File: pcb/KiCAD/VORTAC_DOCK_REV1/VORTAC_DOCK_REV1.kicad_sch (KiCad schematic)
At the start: 31 parts, among them J1 Conn_01x05, J10 Conn_01x03, J2 Conn_01x03, J3 PowerSolderPoint, J4 Conn_01x03, J5 Conn_01x04, J6 Conn_01x04, J7 Conn_01x01, J8 Conn_01x01, J9 Conn_01x03, U1 WS2811, U2 TPS26630RGE, U6 AP63205WU

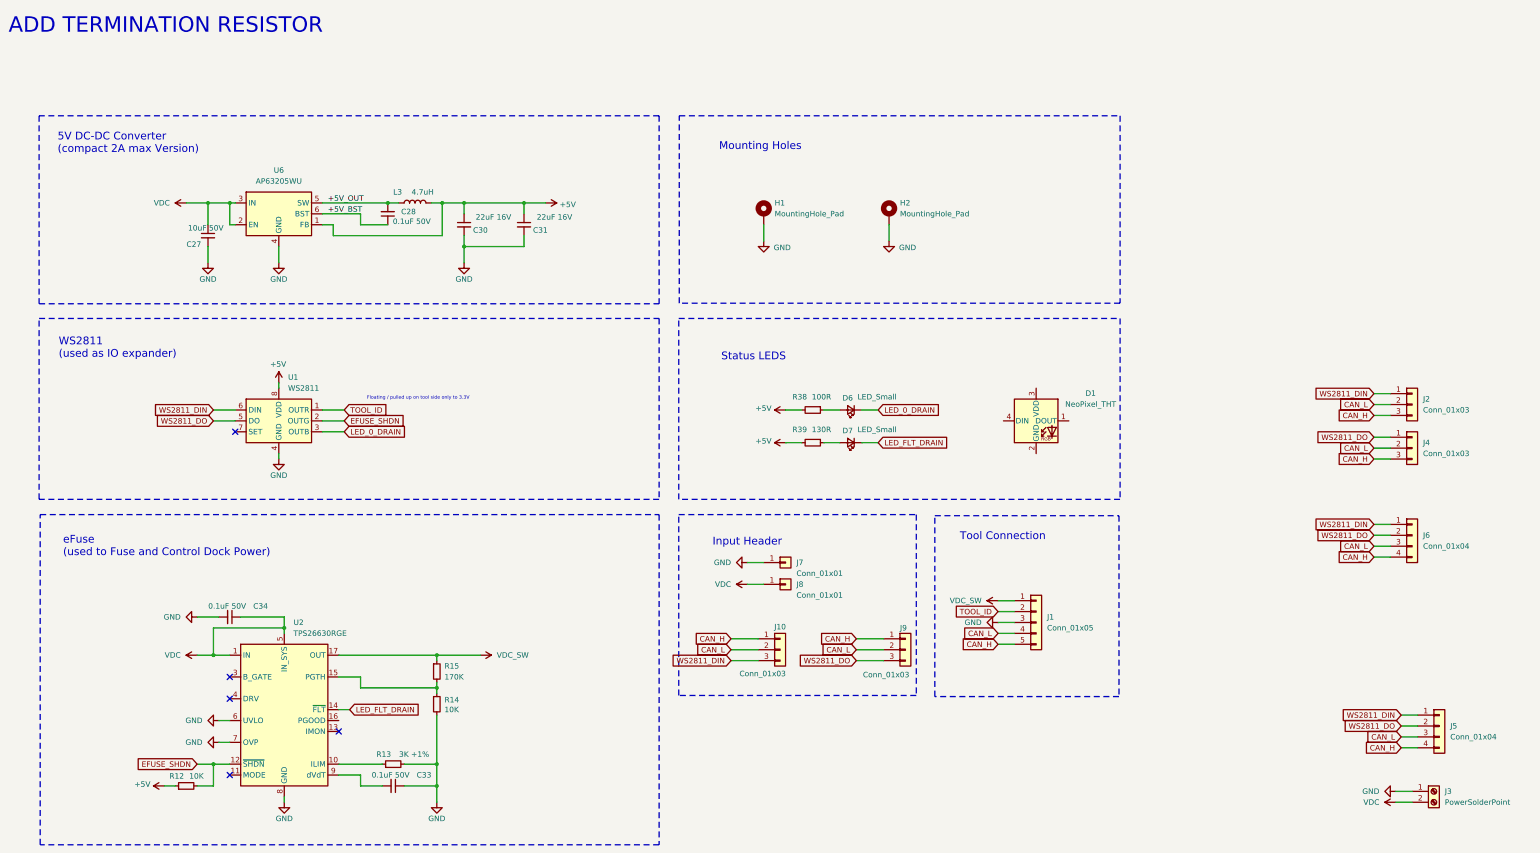
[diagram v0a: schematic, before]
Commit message: Vortac Dock rough component placement #NO-JIRA
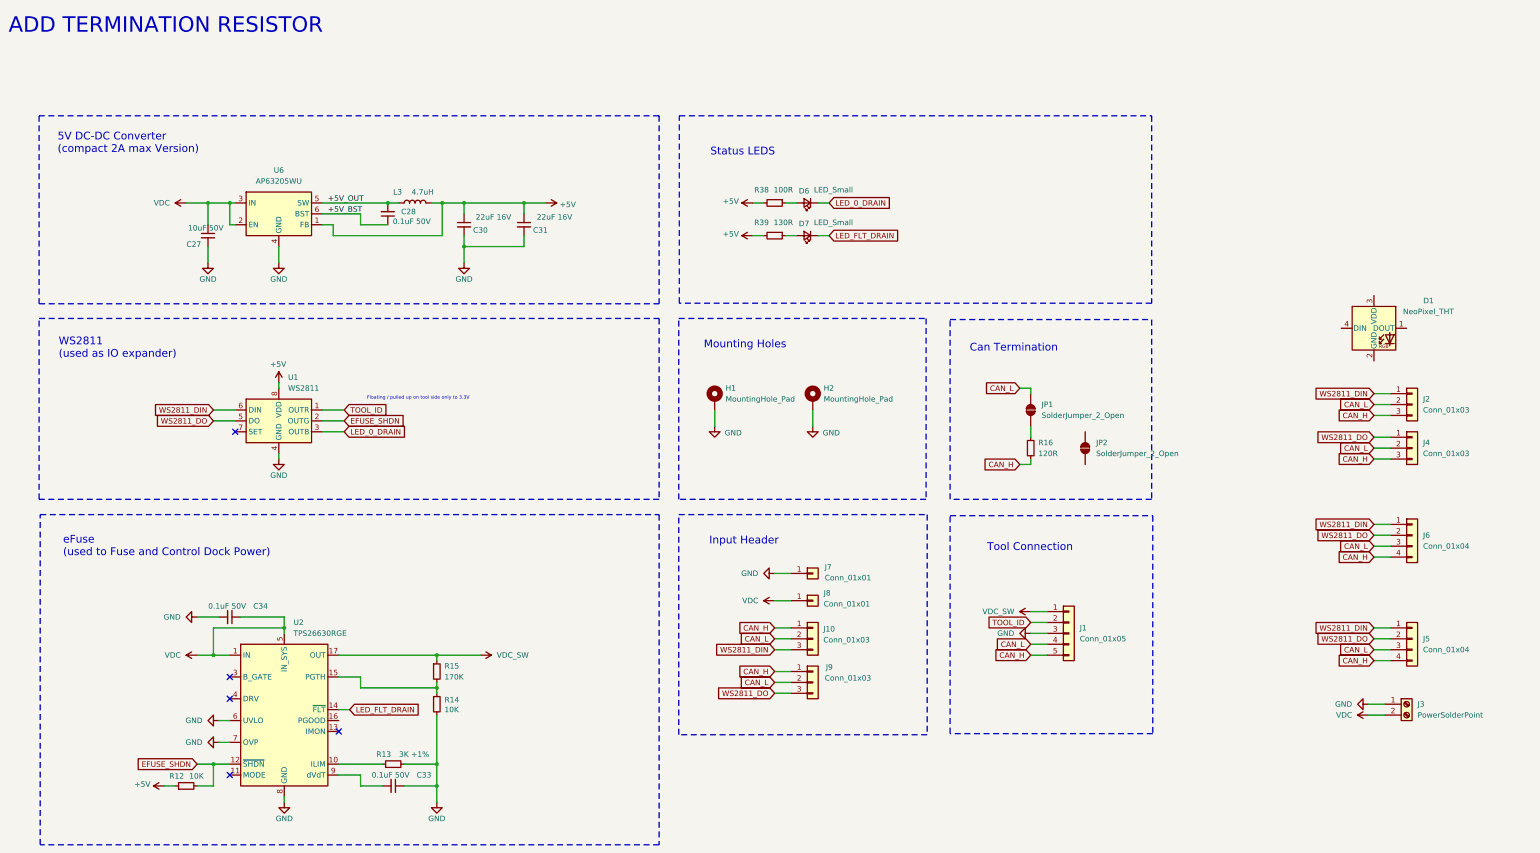
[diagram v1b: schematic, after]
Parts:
- added JP1: SolderJumper_2_Open, Vortac:SolderJumper_Hex_Open_Pad, symbol Jumper:SolderJumper_2_Open
- added JP2: SolderJumper_2_Open, Jumper:SolderJumper-2_P1.3mm_Open_RoundedPad1.0x1.5mm, symbol Jumper:SolderJumper_2_Open
- added R16: 120R, Resistor_SMD:R_0402_1005Metric, symbol Device:R_Small
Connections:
- net CAN_H: now also R16.2
- net CAN_L: now also JP1.2 (B)
- new net: JP1.1 (A), R16.1
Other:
- note added: "Can Termination"
- moved on the sheet: D1, D6, D7, H1, H2, J1, J10, J3, J5, J7, J8, J9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
